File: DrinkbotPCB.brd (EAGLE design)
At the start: 130.8 x 60.6 mm, 35 parts, among them IC1 L7805, J1 POWER_JACKPTH, Q1 MOSFET-NCHANNELFQP30N06L, Q2 MOSFET-NCHANNELFQP30N06L, Q3 MOSFET-NCHANNELFQP30N06L, Q4 MOSFET-NCHANNELFQP30N06L, Q5 MOSFET-NCHANNELFQP30N06L, Q6 MOSFET-NCHANNELFQP30N06L, Q7 MOSFET-NCHANNELFQP30N06L, Q8 MOSFET-NCHANNELFQP30N06L

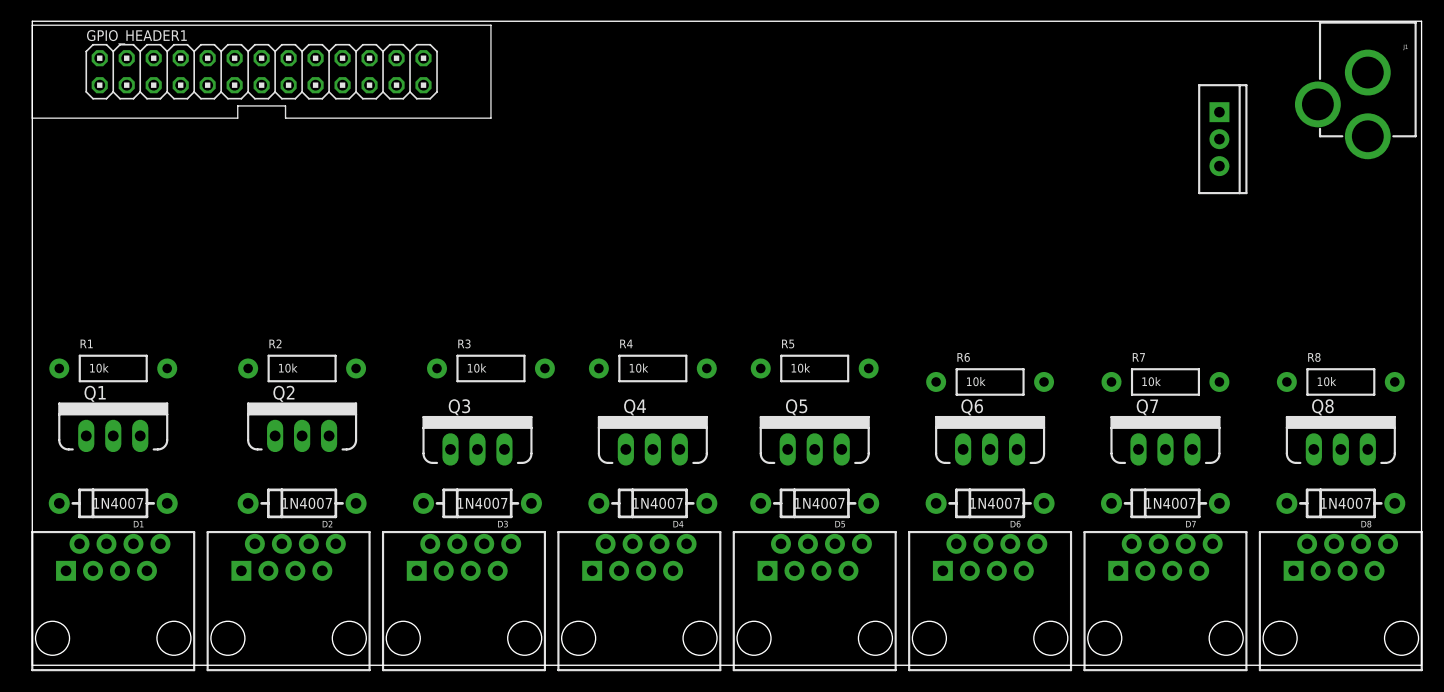
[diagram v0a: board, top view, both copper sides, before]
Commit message: Updated Schematics/Gerbers/Board Layout
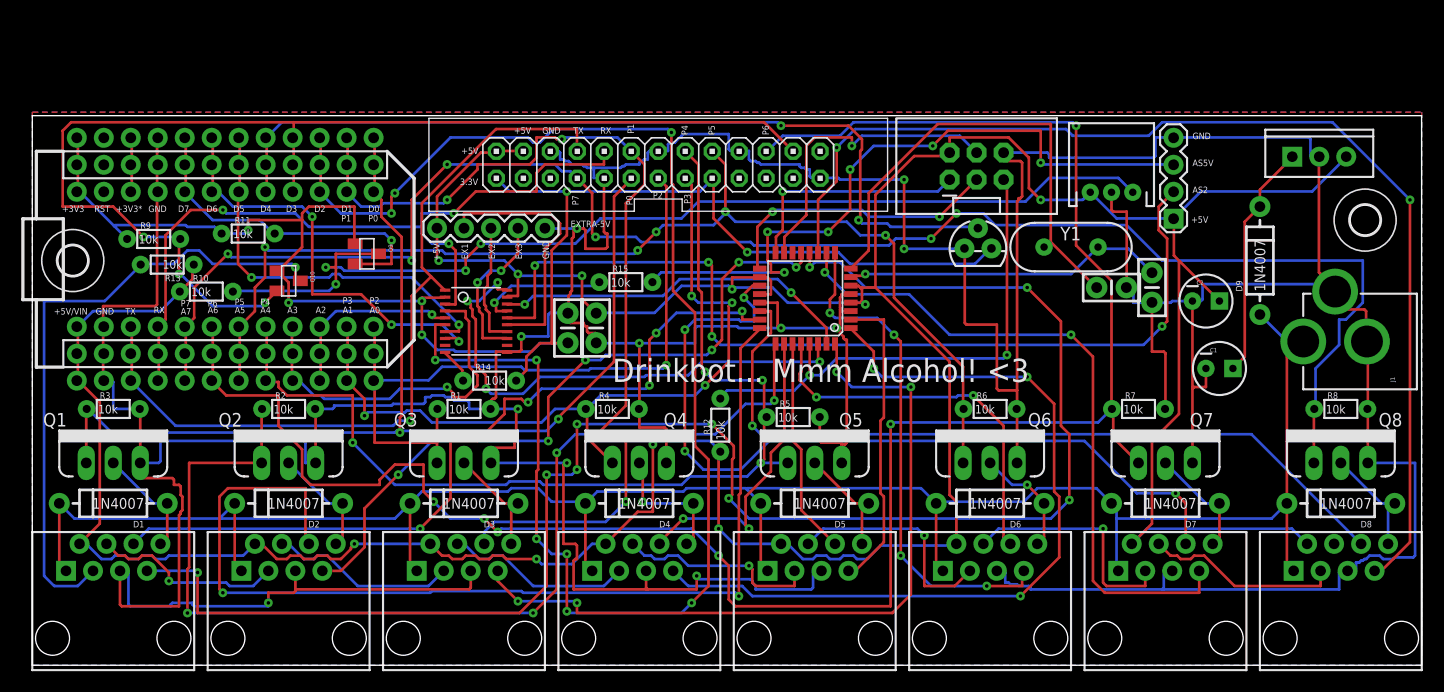
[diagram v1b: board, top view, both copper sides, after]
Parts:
- added C1, C2: 10uF, SparkFun-Passives:CPOL-RADIAL-10UF-25V
- added C3, C4: 22pf, SparkFun-Capacitors:CAP-PTH-SMALL-KIT
- added C5, C6: 0.1uF, SparkFun-Capacitors:CAP-PTH-SMALL-KIT
- added D9: 1N4007, SparkFun-DiscreteSemi:DIODE-1N4001
- added EXTRA-5V: (no value), SparkFun-Connectors:1X05
- added JP1: RGBLED1, SparkFun-Connectors:JST-3-PTH
- added JP3: ISP, SparkFun-Connectors:2X3-SHROUDED
- added JP4: ALCOHOL, SparkFun-Connectors:1X04
- added Q10, Q9: BSS138, SparkFun-DiscreteSemi:SOT23
- added R10, R11, R12, R13, R14, R15, R9: 10k, SparkFun-Resistors:1/6W-RES
- added U$1: SPARK-CORE, Spark:SPARK_CORE_STACKABLE
- added U$2: TMP, SparkFun-Sensors:TO-92
- added U$3, U$7: (no value), holes:2,8
- added U1: ATMEGA328P, SparkFun-DigitalIC:TQFP32-08
- added U2: TXB0108, adafruit:TSSOP20
- added Y1: 16Mhz, SparkFun-FreqCtrl:HC49US
- GPIO_HEADER1: value RPI_GPIO_HEADER -> RPI-GPIO
- IC1: value L7805 -> L7805-5V
- J1: value POWER_JACKPTH -> 12V-PWR
- Q1, Q2, Q3, Q4, Q5, Q6, Q7, Q8: value MOSFET-NCHANNELFQP30N06L -> FQP30N06L
- R1, R2, R3, R4, R5, R6, R7, R8: device SparkFun-Passives:AXIAL-0.4 -> SparkFun-Resistors:1/6W-RES
- moved GPIO_HEADER1 38.4 mm to (58.9, 47.1)
- moved R3 35.8 mm to (7.62, 24.1)
- moved J1 33.9 mm to (133.3, 30.5), turned to 90 degrees
- moved R1 33.2 mm to (40.6, 24.1)
- moved IC1 9.54 mm to (121.2, 47.9), turned to 0 degrees
- moved R4 5.39 mm to (54.6, 24.1)
- moved R5 5.00 mm to (71.6, 23.4)
- moved R2 4.02 mm to (24.1, 24.1)
- moved R7 3.59 mm to (104.1, 24.1)
- moved Q2 2.84 mm to (24.1, 19.1)
- moved R6 2.54 mm to (90.2, 24.1)
- moved R8 2.54 mm to (123.2, 24.1)
- moved Q1 2.54 mm to (7.62, 19.1)
- moved Q4 1.80 mm to (57.1, 19.1)
- moved Q3 1.80 mm to (40.6, 19.1)
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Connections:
- new net AP0: U1.23, UNIT0.6
- new net AP1: U1.24, UNIT1.6
- new net AP2: U1.25, UNIT2.6
- new net AP3: U1.26, UNI3.6
- new net AP4: U1.27, UNIT4.6
- new net AP5: U1.28, UNIT5.6
- new net AP6: U1.19, UNIT6.6
- new net AP7: U1.22, UNIT7.6
- new net AS2-3V: U$1.#10, U$1.10, U$1.@10, U2.5
- new net AS2-5V: JP4.2, U2.16
- new net AS3V: U$1.#9, U$1.9, U$1.@9, U2.4
- new net AS5V: R15.1, U2.17
- new net AT-RX: U1.30, U2.20
- new net AT-TX: U1.31, U2.18
- new net DP0: U1.12, UNIT0.7
- new net DP1: U1.13, UNIT1.7
- new net DP2: U1.32, UNIT2.7
- new net DP3: U1.1, UNI3.7
- new net DP4: U1.2, UNIT4.7
- new net DP5: U1.9, UNIT5.7
- new net DP6: U1.10, UNIT6.7
- new net DP7: U1.11, UNIT7.7
- new net EXTRA1-3V3: U$1.#15, U$1.15, U$1.@15, U2.6
- new net EXTRA1-5V: EXTRA-5V.4, U2.15
- new net EXTRA2-3V3: U$1.#18, U$1.18, U$1.@18, U2.7
- new net EXTRA2-5V: EXTRA-5V.3, U2.14
- new net EXTRA3-3V3: U$1.#19, U$1.19, U$1.@19, U2.8
- new net EXTRA3-5V: EXTRA-5V.2, U2.13
- new net HV1: JP1.3, Q9.3, R10.2
- new net LEDIN0: Q10.3, R13.2, UNIT0.3
- new net LEDOUT0: UNIT0.4, UNIT1.3
- new net LEDOUT1: UNIT1.4, UNIT2.3
- new net LEDOUT2: UNI3.3, UNIT2.4
- new net LEDOUT3: UNI3.4, UNIT4.3
- new net LEDOUT4: UNIT4.4, UNIT5.3
- new net LEDOUT5: UNIT5.4, UNIT6.3
- new net LEDOUT6: UNIT6.4, UNIT7.3
- new net LEDOUT7: UNIT7.4
- new net LV-RX: GPIO_HEADER1.10, U$1.#4, U$1.4, U$1.@4, U2.3
- new net LV-TX: GPIO_HEADER1.8, U$1.#3, U$1.3, U$1.@3, U2.1
- new net MISO: JP3.1, U1.16
- new net MOSI: JP3.4, U1.15
- new net N$1: C1.1, D9.C, IC1.IN
- new net N$2: C3.2, U1.7, Y1.2
- new net N$3: C4.2, U1.8, Y1.1
- new net N$5: R14.2, U2.10
- new net N$7: JP4.3, R15.2
- new net PUMPLEDS: GPIO_HEADER1.24, Q10.2, R9.2, U$1.#16, U$1.16, U$1.@16
- new net RESET: JP3.5, R12.2, U1.29
- new net RGBLED1: Q9.2, R11.2, U$1.#20, U$1.20, U$1.@20
- new net SCK: JP3.3, U1.17
- new net TEMPSENSOR1: U$1.#17, U$1.17, U$1.@17, U$2.2
- new net VDDA: U$1.#22, U$1.22, U$1.@22
- net +3V3: now also C6.1, Q10.1, Q9.1, R11.1, R14.1, R9.1, U$1.#24, U$1.24, U$1.@24, U$2.3, U2.2
- net +5V: now also C2.1, C5.1, EXTRA-5V.5, JP1.1, JP3.2, JP4.1, R10.1, R12.1, R13.1, U$1.#1, U$1.1, U$1.@1, U1.18, U1.20, U1.4, U1.6, U2.19, UNI3.2, UNIT0.2, UNIT1.2, UNIT2.2, UNIT4.2, UNIT5.2, UNIT6.2, UNIT7.2
- net GND: now also C1.2, C2.2, C3.1, C4.1, C5.2, C6.2, EXTRA-5V.1, JP1.2, JP3.6, JP4.4, R1.2, R2.2, R3.2, R4.2, R5.2, R6.2, R7.2, R8.2, U$1.#2, U$1.#21, U$1.2, U$1.21, U$1.@2, U$1.@21, U$2.1, U1.21, U1.3, U1.5, U2.11, UNI3.5, UNIT0.5, UNIT1.5, UNIT2.5, UNIT4.5, UNIT5.5, UNIT6.5, UNIT7.5; no longer R1.P$2, R2.P$2, R3.P$2, R4.P$2, R5.P$2, R6.P$2, R7.P$2, R8.P$2
- net PUMP0: now also R3.1, U$1.#13, U$1.13, U$1.@13; no longer R1.P$1
- net PUMP1: now also R2.1, U$1.#14, U$1.14, U$1.@14; no longer R2.P$1
- net PUMP2: now also R1.1, U$1.#12, U$1.12, U$1.@12; no longer R3.P$1
- net PUMP3: now also R4.1, U$1.#11, U$1.11, U$1.@11; no longer R4.P$1
- net PUMP4: now also R5.1, U$1.#8, U$1.8, U$1.@8; no longer R5.P$1
- net PUMP5: now also R6.1, U$1.#7, U$1.7, U$1.@7; no longer R6.P$1
- net PUMP6: now also R7.1, U$1.#6, U$1.6, U$1.@6; no longer R7.P$1
- net PUMP7: now also R8.1, U$1.#5, U$1.5, U$1.@5; no longer R8.P$1
- net VIN12: now also D9.A; no longer IC1.IN
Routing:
- net GND: track 0.00 -> 613.6 mm, vias 0 -> 11
- net +5V: track 0.00 -> 367.0 mm, vias 0 -> 10
- net VIN12: track 0.00 -> 199.4 mm
- net PUMP6: track 0.00 -> 189.9 mm, vias 0 -> 6
- net DP0: track 0.00 -> 159.4 mm, vias 0 -> 9
- net +3V3: track 0.00 -> 158.5 mm, vias 0 -> 6
- net PUMP7: track 0.00 -> 157.9 mm, vias 0 -> 6
- net PUMP1: track 0.00 -> 145.6 mm, vias 0 -> 6
- net EXTRA1-3V3: track 0.00 -> 142.2 mm, vias 0 -> 9
- net PUMPLEDS: track 0.00 -> 110.9 mm, vias 0 -> 3
- net PUMP5: track 0.00 -> 105.9 mm, vias 0 -> 5
- net DP7: track 0.00 -> 105.8 mm, vias 0 -> 2
- net PUMP0: track 0.00 -> 105.7 mm, vias 0 -> 2
- net HV1: track 0.00 -> 98.8 mm, vias 0 -> 4
- net PUMP4: track 0.00 -> 98.2 mm, vias 0 -> 4
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- added copper zone on layer 1, net GND
- added copper zone on layer 16, net GND
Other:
- board size 130.8 x 60.6 mm -> 130.8 x 51.7 mm
- board text added: "+"
- board text added: "+3V3"
- board text added: "+3V3*"
- board text added: "+5V"
- board text added: "+5V/VIN"
- board text added: "0.1uF"
- board text added: "22pf"
- board text added: "3.3V"
- board text added: "A0"
- board text added: "A1"
- board text added: "A2"
- board text added: "A3"
- board text added: "A4"
- board text added: "A5"
- board text added: "A6"
- board text added: "A7"
- board text added: "AS2"
- board text added: "AS5V"
- board text added: "ATMEGA328P"
- board text added: "Copyright 2015"
- board text added: "D0"
- board text added: "D1"
- board text added: "D2"
- board text added: "D3"
- board text added: "D4"
- board text added: "D5"
- board text added: "D6"
- board text added: "D7"
- board text added: "Design by Felix"
- board text added: "Drinkbot Prototype 1.0"
- board text added: "Drinkbot... Mmm Alcohol! <3"
- board text added: "EX1"
- board text added: "EX2"
- board text added: "EX3"
- board text added: "GND"
- board text added: "L7805-5V"
- board text added: "P0"
- board text added: "P1"
- board text added: "P2"
- board text added: "P3"
- board text added: "P4"
- board text added: "P5"
- board text added: "P6"
- board text added: "P7"
- board text added: "RST"
- board text added: "RX"
- board text added: "TX"
